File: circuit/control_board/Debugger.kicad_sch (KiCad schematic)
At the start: 6 parts, among them M1 Debugger, SW1 SW_DIP_x02, U10 CH440R

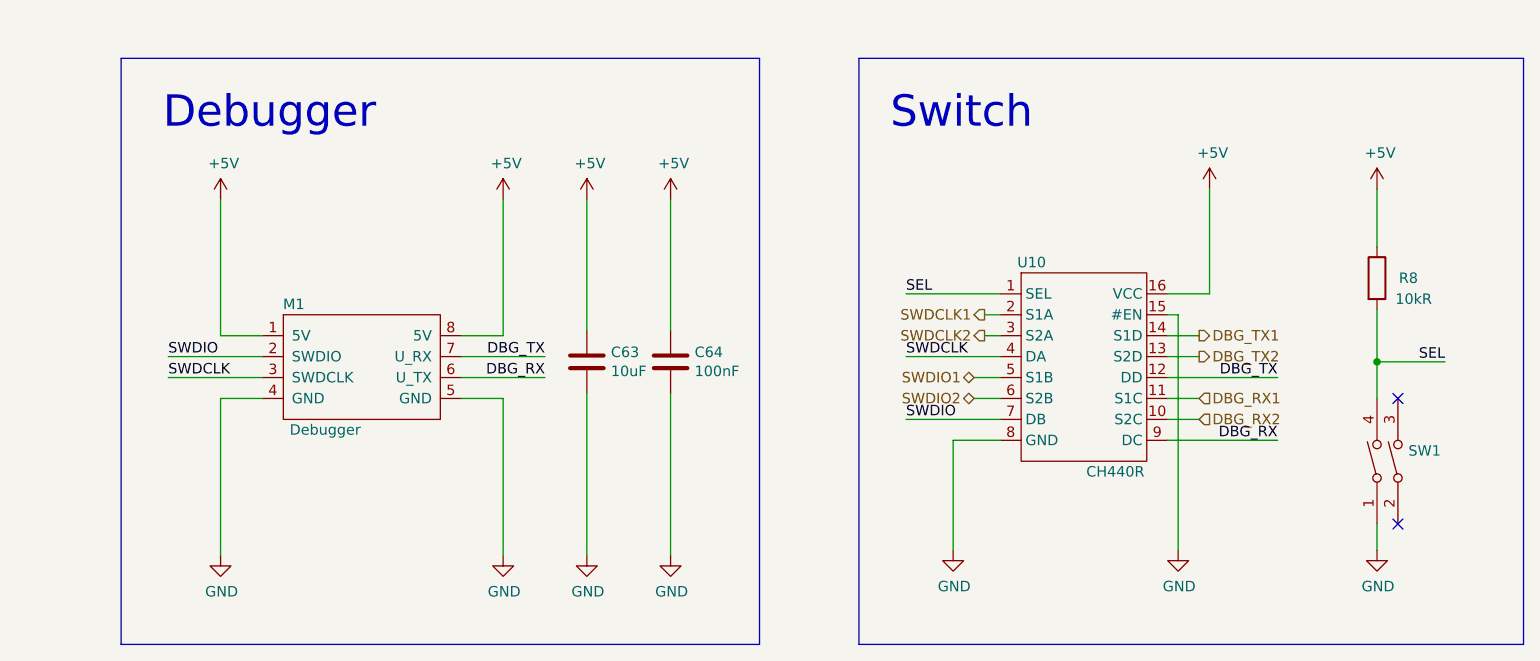
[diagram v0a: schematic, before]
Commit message: Modify the main control board schematic, replace the IMU device and remove the isolation module.
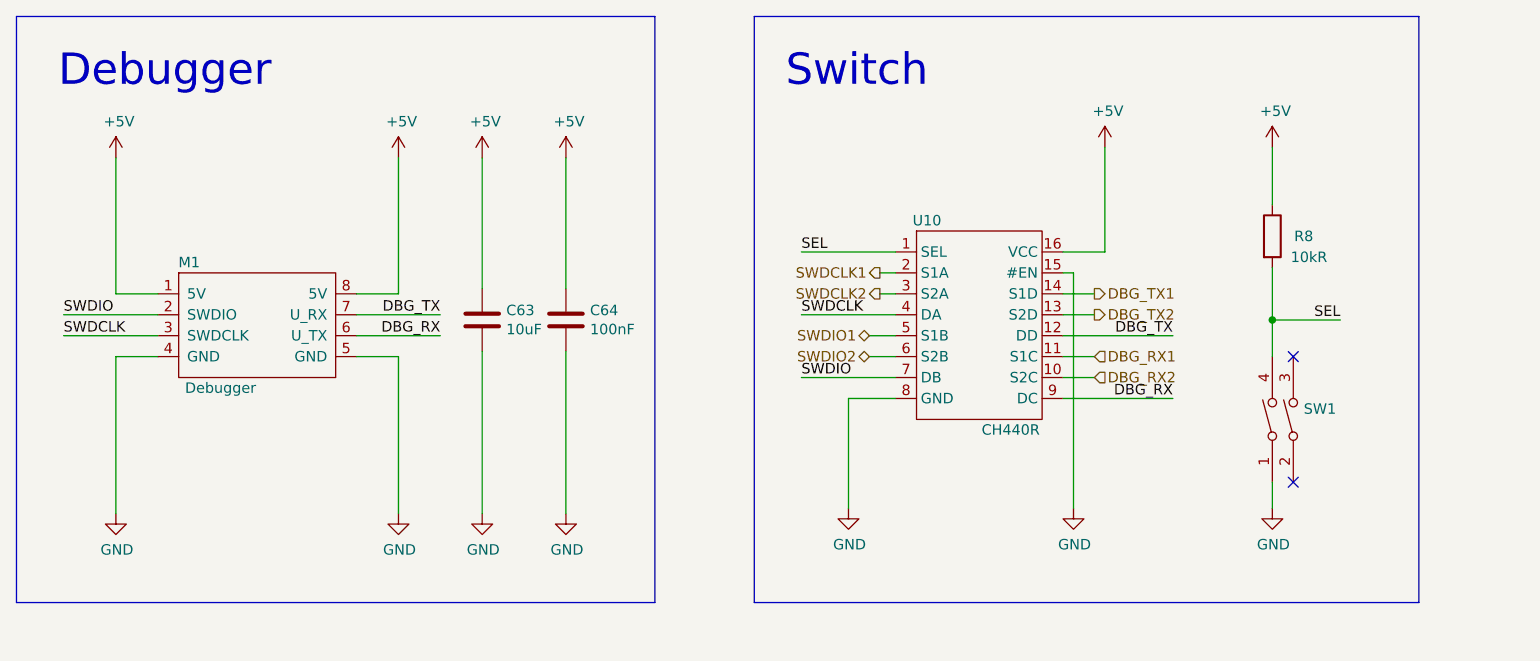
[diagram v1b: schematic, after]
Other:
- moved on the sheet: C63, C64, M1, R8, SW1, U10
